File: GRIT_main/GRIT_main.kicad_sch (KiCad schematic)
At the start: 1 part, among them J1 Raspberry_Pi_4

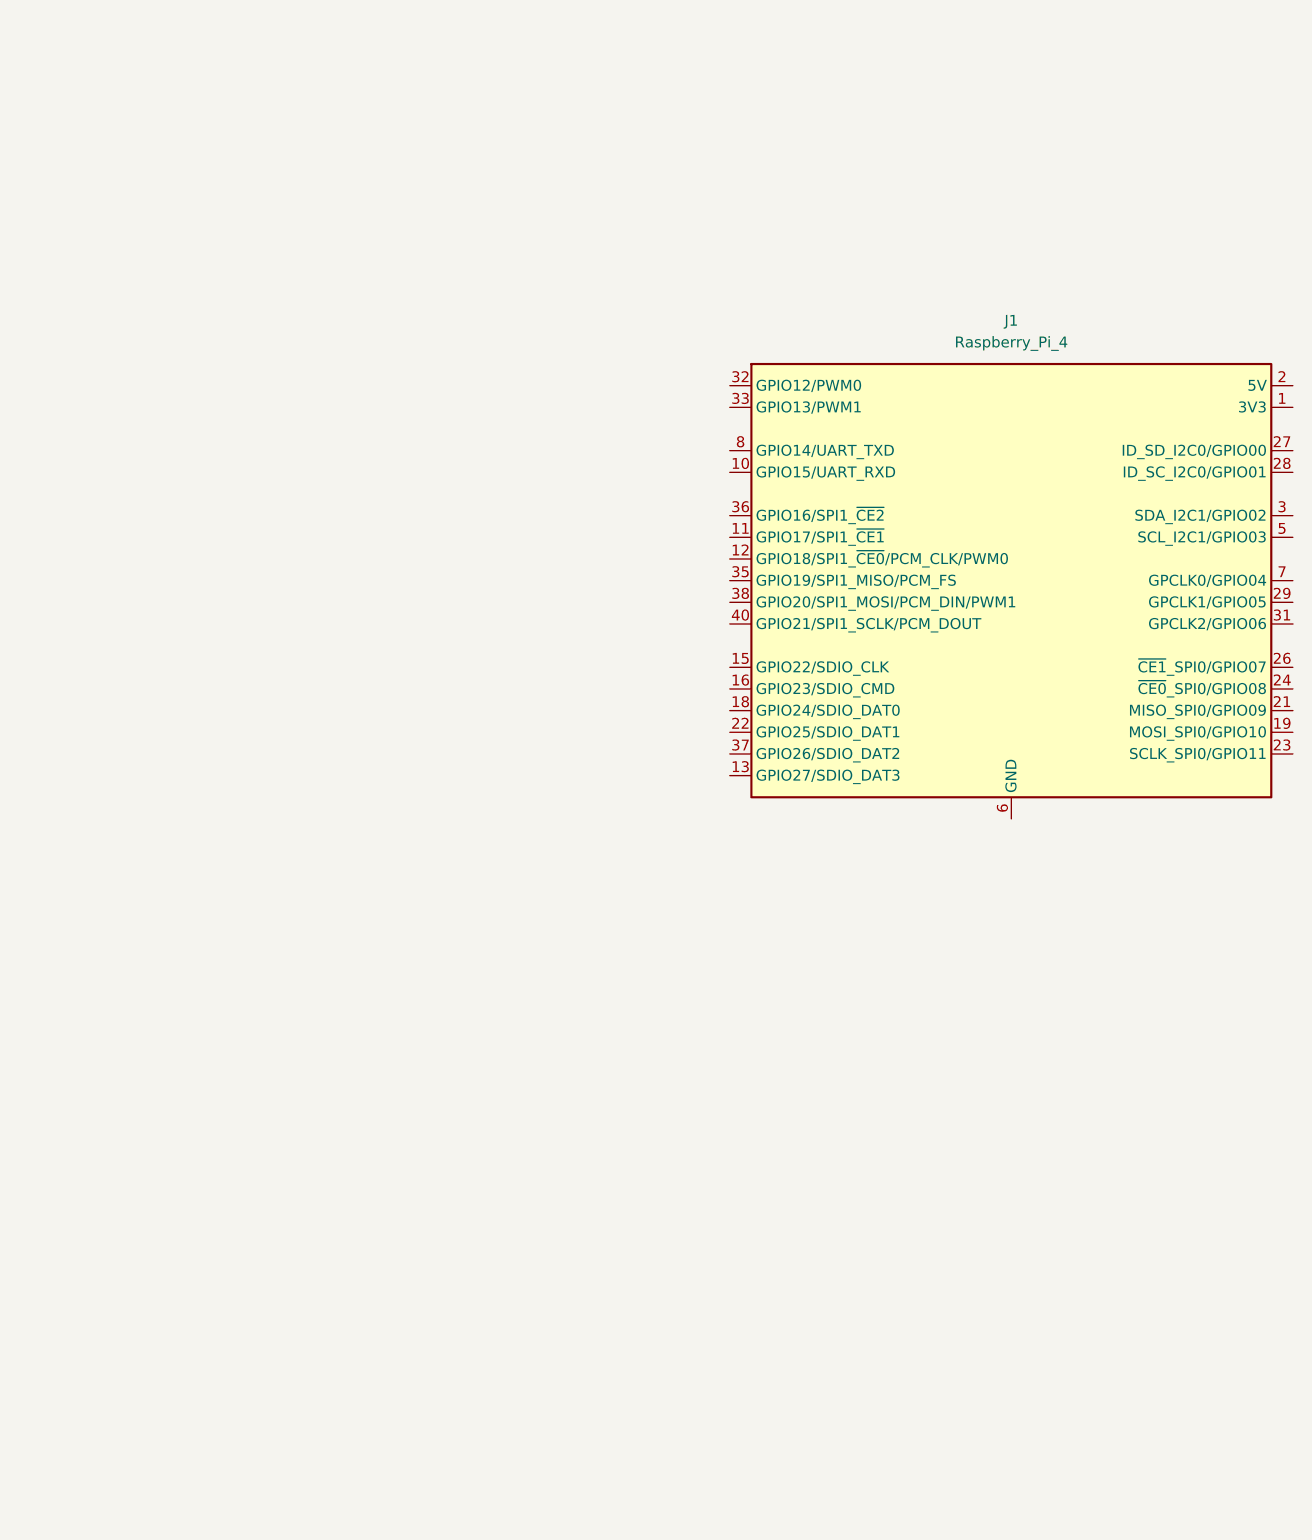
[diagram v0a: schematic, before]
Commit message: Updated Schematic
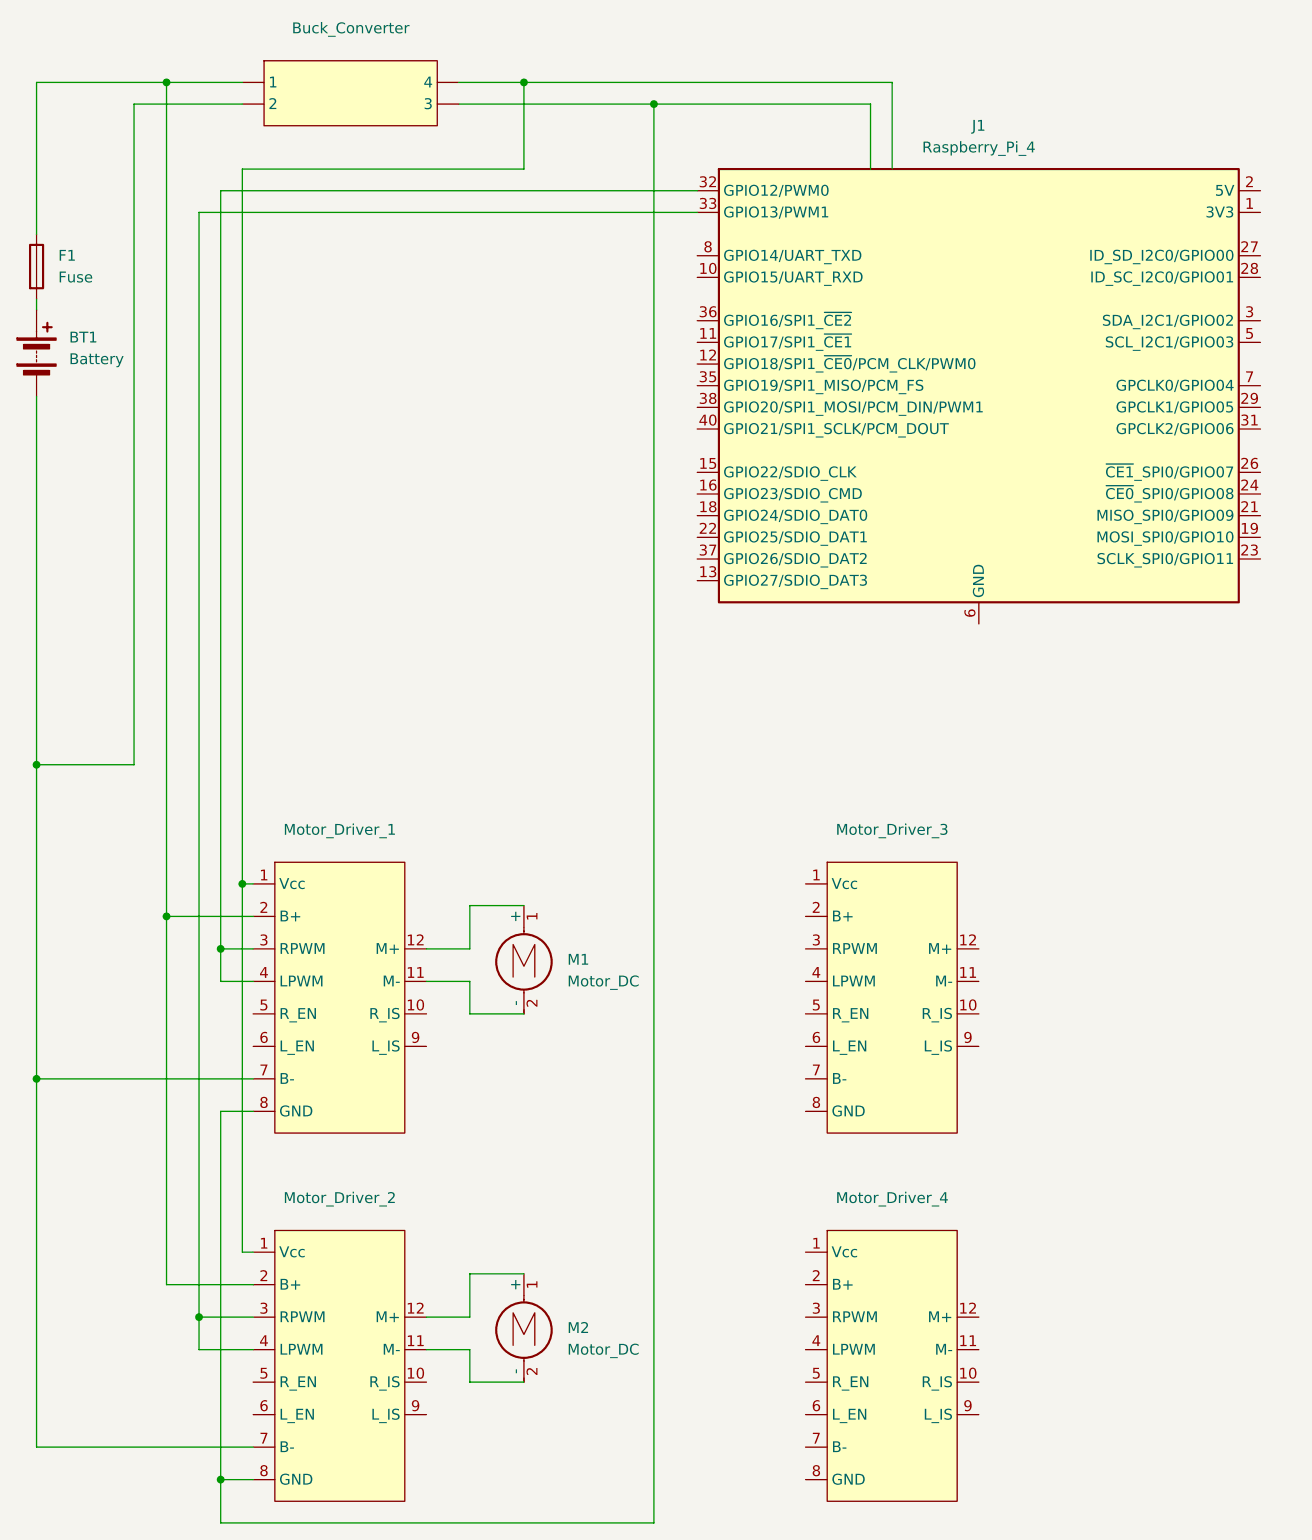
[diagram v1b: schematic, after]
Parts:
- added BT1: Battery, symbol Device:Battery
- added Buck_Converter: ~, symbol Custom_Symbols:Buck_Converter_12V_to_5V
- added F1: Fuse, symbol Device:Fuse
- added M1, M2: Motor_DC, symbol Motor:Motor_DC
- added Motor_Driver_1, Motor_Driver_2, Motor_Driver_3, Motor_Driver_4: ~, symbol Custom_Symbols:12V_Motor_Controller
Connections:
- net at J1.32 (GPIO12/PWM0): now also Motor_Driver_1.3 (RPWM), Motor_Driver_1.4 (LPWM)
- net at J1.33 (GPIO13/PWM1): now also Motor_Driver_2.3 (RPWM), Motor_Driver_2.4 (LPWM)
- new net: Buck_Converter. (4), F1.1, Motor_Driver_1.2 (B+), Motor_Driver_2.2 (B+)
- new net: Buck_Converter. (4), Motor_Driver_1.1 (Vcc), Motor_Driver_2.1 (Vcc)
- new net: BT1.2 (-), Buck_Converter. (4), Motor_Driver_1.7 (B-), Motor_Driver_2.7 (B-)
- new net: Buck_Converter. (4), Motor_Driver_1.8 (GND), Motor_Driver_2.8 (GND)
- new net: M2.1 (+), Motor_Driver_2.12 (M+)
- new net: M2.2 (-), Motor_Driver_2.11 (M-)
- new net: BT1.1 (+), F1.2
- new net: M1.1 (+), Motor_Driver_1.12 (M+)
- new net: M1.2 (-), Motor_Driver_1.11 (M-)
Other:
- moved on the sheet: J1
